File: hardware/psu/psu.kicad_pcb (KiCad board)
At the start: 2 copper layers, 165.1 x 95.2 mm, 56 parts, among them J1 Conn_01x02, J10 Conn_01x04, J11 Conn_01x03, J12 Conn_01x02, J13 Conn_01x03, J2 Conn_01x05, J3 Conn_01x02, J4 Conn_01x06, J5 Conn_01x03, J6 Conn_01x05, J7 Conn_01x08, J8 Conn_01x03, J9 Conn_01x04, SW1 SW_SPST, U1 LM7905_TO220

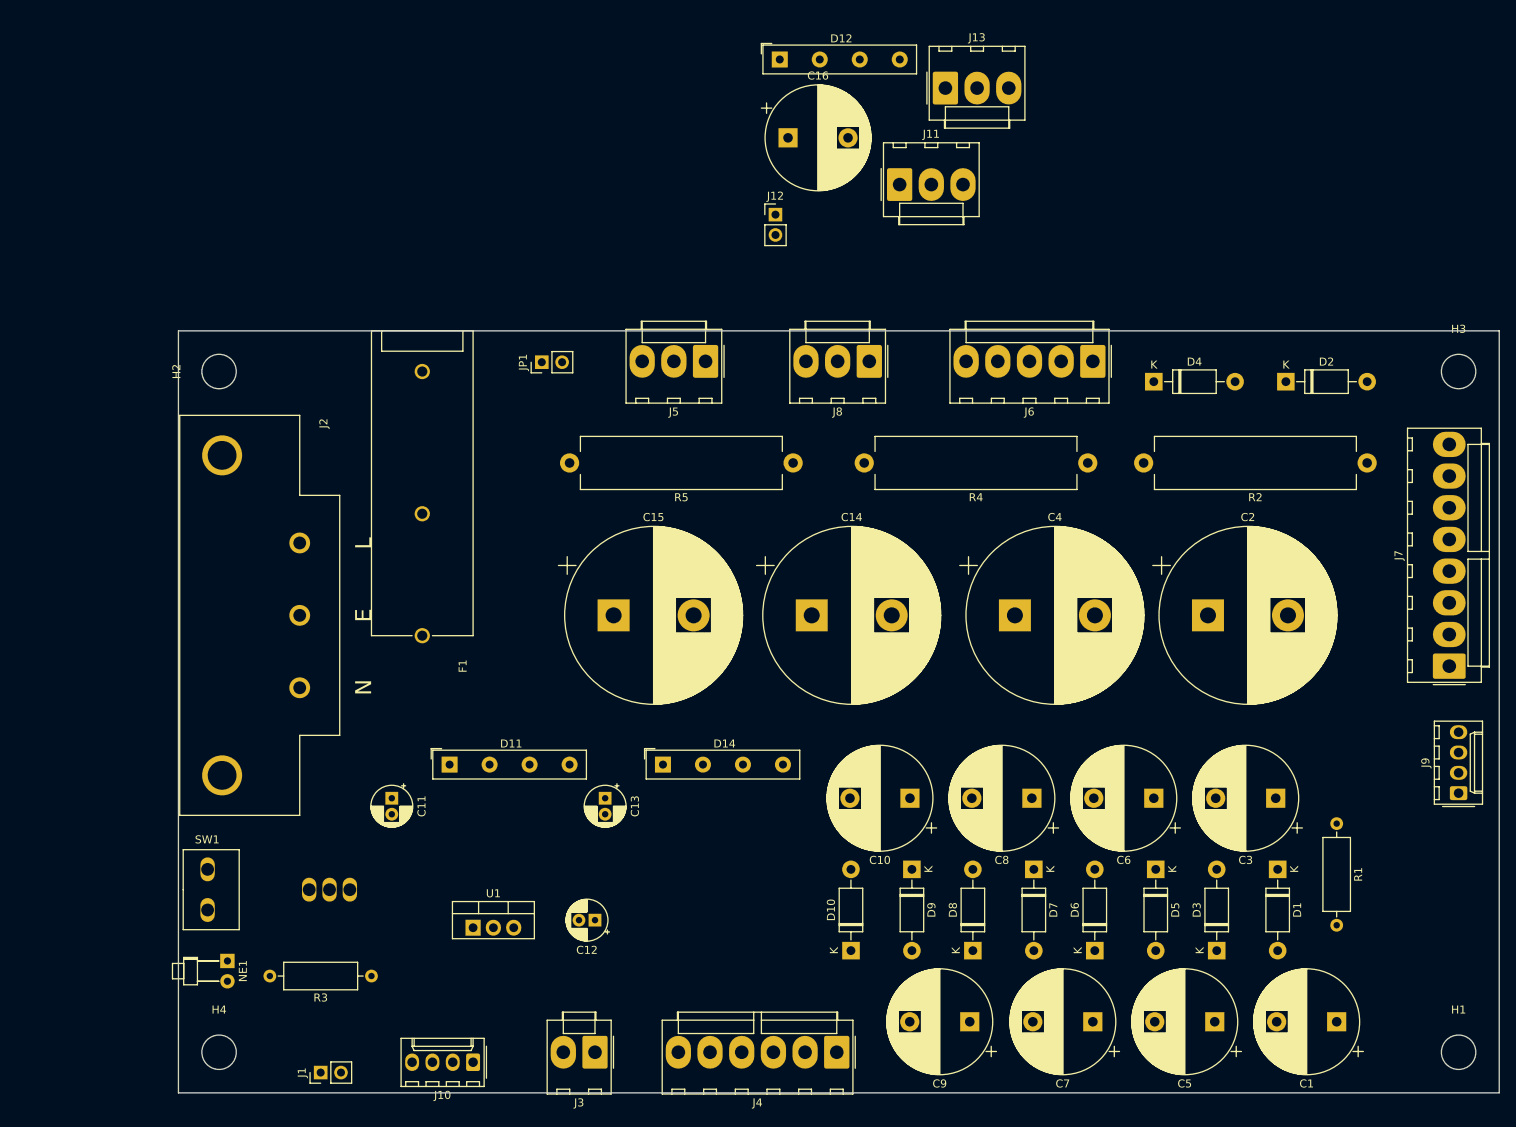
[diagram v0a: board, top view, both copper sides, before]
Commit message: working on chassis layout
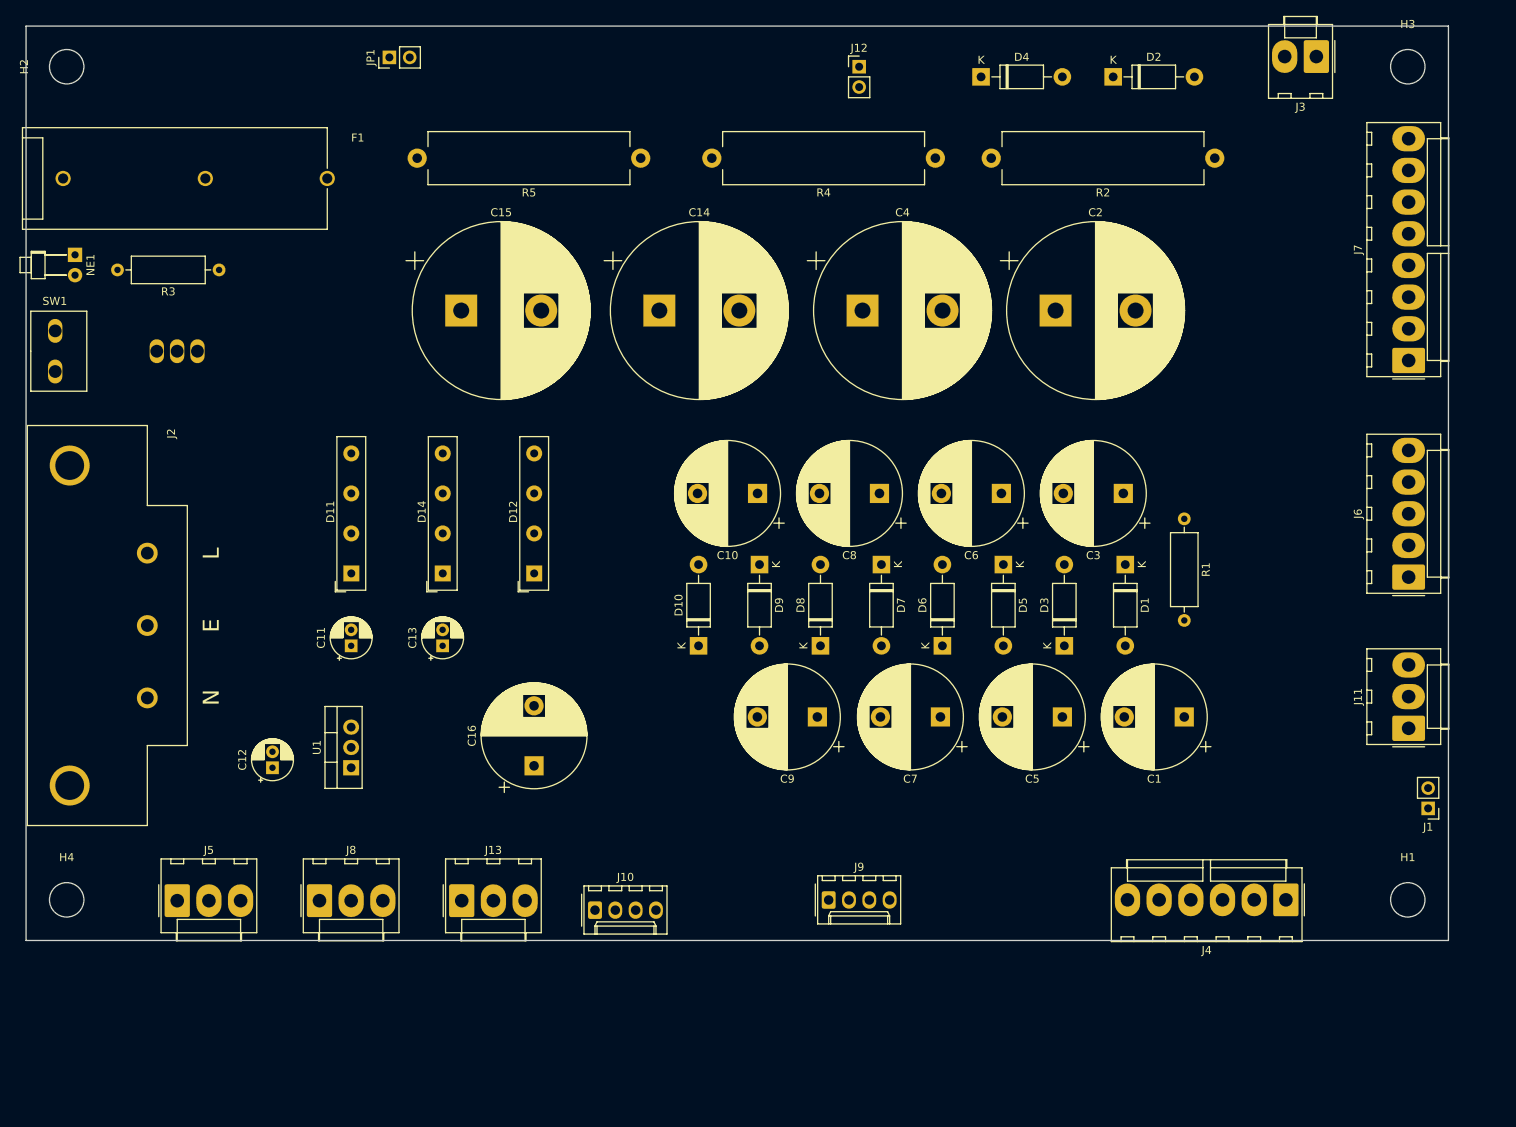
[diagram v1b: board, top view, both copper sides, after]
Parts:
- moved J3 153.7 mm to (186.7, 29.2)
- moved J1 142.3 mm to (200.7, 123.2), turned to 180 degrees
- moved J13 118.2 mm to (79.9, 134.7)
- moved J8 96.3 mm to (62.1, 134.7), turned to 0 degrees
- moved J5 94.4 mm to (44.3, 134.7), turned to 0 degrees
- moved J11 93.1 mm to (198.2, 113.2), turned to 90 degrees
- moved R3 90.3 mm to (49.5, 55.9)
- moved NE1 90.3 mm to (31.5, 54.0)
- moved C16 84.7 mm to (88.9, 117.9), turned to 90 degrees
- moved J9 79.9 mm to (125.7, 134.6), turned to 0 degrees
- moved D12 71.2 mm to (88.9, 93.8), turned to 90 degrees
- moved SW1 70.0 mm to (41.7, 66.0)
- moved J4 59.3 mm to (182.9, 134.6)
- moved F1 58.4 mm to (63.1, 44.5), turned to 0 degrees
- moved J6 47.8 mm to (198.2, 94.3), turned to 90 degrees
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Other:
- board size 165.1 x 95.2 mm -> 177.8 x 114.3 mm
